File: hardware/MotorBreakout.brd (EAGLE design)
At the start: 160 x 100 mm, 1 part

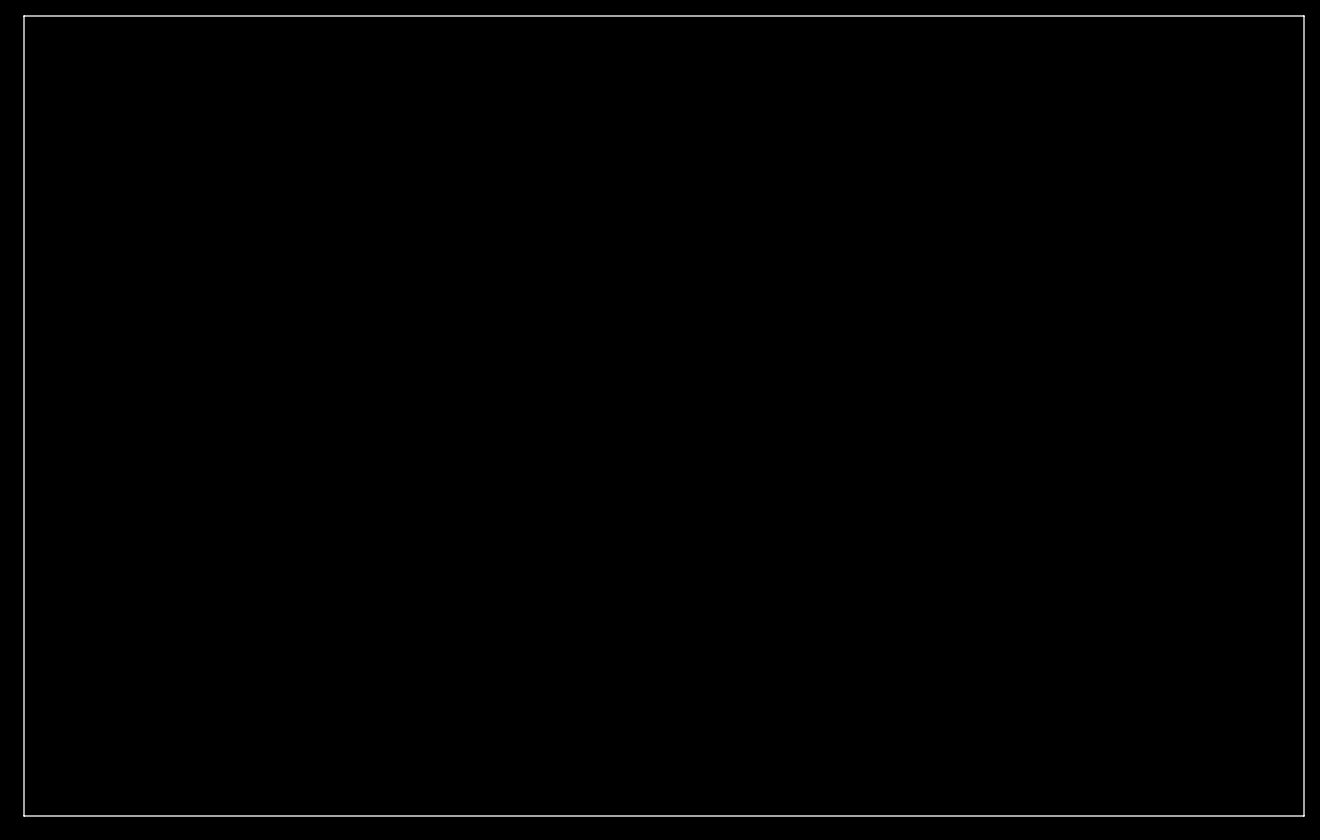
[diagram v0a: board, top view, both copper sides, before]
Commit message: Basic breakout complete.y
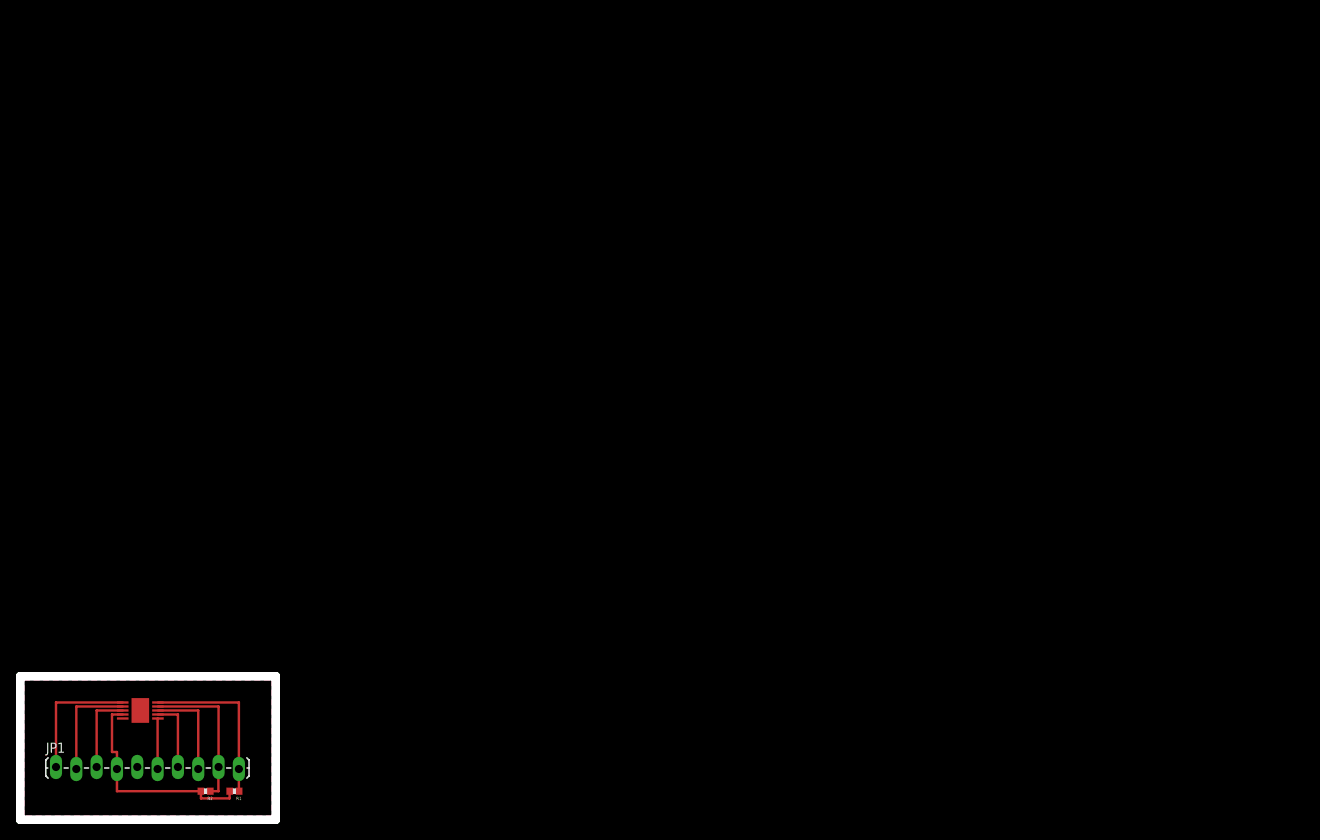
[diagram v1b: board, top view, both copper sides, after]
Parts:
- added JP1: (no value), SparkFun-Connectors:1X10_LOCK_LONGPADS
- added R1, R2: 4.7k, SparkFun-Resistors:0402-RES
- added U$1: DRV8830, DRV8830:DRV8830
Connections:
- new net !FAULT: JP1.6, U$1.P$6
- new net 3.3V: JP1.4, R1.2, R2.2, U$1.P$4
- new net A0: JP1.7, U$1.P$7
- new net A1: JP1.8, U$1.P$8
- new net GND: JP1.5, U$1.P$11, U$1.P$5
- new net ISENSE: JP1.2, U$1.P$2
- new net OUT1: JP1.3, U$1.P$3
- new net OUT2: JP1.1, U$1.P$1
- new net SCL: JP1.10, R1.1, U$1.P$10
- new net SDA: JP1.9, R2.1, U$1.P$9
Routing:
- net 3.3V: track 0.00 -> 27.4 mm
- net SCL: track 0.00 -> 21.2 mm
- net SDA: track 0.00 -> 19.2 mm
- net OUT2: track 0.00 -> 16.4 mm
- net ISENSE: track 0.00 -> 13.6 mm
- net A1: track 0.00 -> 12.4 mm
- net OUT1: track 0.00 -> 10.3 mm
- net A0: track 0.00 -> 9.06 mm
- net !FAULT: track 0.00 -> 6.36 mm
- added copper zone on layer 1, net GND
- added copper zone on layer 16, net GND
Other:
- board size 160 x 100 mm -> 32 x 18 mm
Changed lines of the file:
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@@
 <setting verticaltext="up"/>
 </settings>
-<grid distance="0.05" unitdist="inch" unit="inch" style="lines" multiple="1" display="no" altdistance="0.025" altunitdist="inch" altunit="inch"/>
+<grid distance="0.5" unitdist="mm" unit="mm" style="lines" multiple="1" display="yes" altdistance="0.1" altunitdist="mm" altunit="mm"/>
 <layers>
 <layer number="1" name="Top" color="4" fill="1" visible="yes" active="yes"/>
@@
 <layer number="44" name="Drills" color="7" fill="1" visible="no" active="yes"/>
 <layer number="45" name="Holes" color="7" fill="1" visible="no" active="yes"/>
-<layer number="46" name="Milling" color="3" fill="1" visible="no" active="yes"/>
+<layer number="46" name="Milling" color="3" fill="1" visible="yes" active="yes"/>
 <layer number="47" name="Measures" color="7" fill="1" visible="no" active="yes"/>
 <layer number="48" name="Document" color="7" fill="1" visible="yes" active="yes"/>
@@
 <layer number="113" name="IDFDebug" color="4" fill="1" visible="yes" active="yes"/>
 <layer number="116" name="Patch_BOT" color="9" fill="4" visible="yes" active="yes"/>
+<layer number="118" name="Rect_Pads" color="7" fill="1" visible="yes" active="yes"/>
 <layer number="121" name="_tsilk" color="7" fill="1" visible="yes" active="yes"/>
 <layer number="122" name="_bsilk" color="7" fill="1" visible="yes" active="yes"/>
@@
 <board>
 <plain>
-<wire x1="0" y1="0" x2="160" y2="0" width="0" layer="20"/>
-<wire x1="160" y1="0" x2="160" y2="100" width="0" layer="20"/>
-<wire x1="160" y1="100" x2="0" y2="100" width="0" layer="20"/>
-<wire x1="0" y1="100" x2="0" y2="0" width="0" layer="20"/>
+<wire x1="0" y1="0" x2="31" y2="0" width="0" layer="20"/>
+<wire x1="31" y1="0" x2="31" y2="17" width="0" layer="20"/>
+<wire x1="31" y1="17" x2="0" y2="17" width="0" layer="20"/>
+<wire x1="0" y1="17" x2="0" y2="0" width="0" layer="20"/>
+<wire x1="-0.5" y1="17.5" x2="31.5" y2="17.5" width="1" layer="46"/>
+<wire x1="31.5" y1="17.5" x2="31.5" y2="-0.5" width="1" layer="46"/>
+<wire x1="31.5" y1="-0.5" x2="-0.5" y2="-0.5" width="1" layer="46"/>
+<wire x1="-0.5" y1="-0.5" x2="-0.5" y2="17.5" width="1" layer="46"/>
 </plain>
 <attributes>
@@
 <attribute name="DESIGNER" value="Nobody" x="0" y="0" size="1.778" layer="27" display="off"/>
 </element>
+<element name="U$1" library="DRV8830" package="DRV8830" value="DRV8830" x="14.54" y="13.19"/>
+<element name="JP1" library="SparkFun-Connectors" package="1X10_LOCK_LONGPADS" value="" x="4" y="6"/>
+<element name="R1" library="SparkFun-Resistors" package="0402-RES" value="4.7k" x="26.3" y="3.1" rot="R180"/>
+<element name="R2" library="SparkFun-Resistors" package="0402-RES" value="4.7k" x="22.7" y="3.1" rot="R180"/>
 </elements>
 <signals>
+<signal name="3.3V">
+<contactref element="U$1" pad="P$4"/>
+<contactref element="JP1" pad="4"/>
+<wire x1="12.34" y1="12.69" x2="11" y2="12.69" width="0.3048" layer="1"/>
+<wire x1="11" y1="12.69" x2="11" y2="8" width="0.3048" layer="1"/>
+<wire x1="11" y1="8" x2="11.62" y2="8" width="0.3048" layer="1"/>
+<wire x1="11.62" y1="8" x2="11.62" y2="5.873" width="0.3048" layer="1"/>
+<contactref element="R1" pad="2"/>
+<contactref element="R2" pad="2"/>
+<wire x1="22.12" y1="3.1" x2="11.62" y2="3.1" width="0.3048" layer="1"/>
+<wire x1="11.62" y1="3.1" x2="11.62" y2="5.873" width="0.3048" layer="1"/>
+<wire x1="25.72" y1="3.1" x2="25.7" y2="3.1" width="0.3048" layer="1"/>
+<wire x1="25.7" y1="3.1" x2="25.7" y2="2.2" width="0.3048" layer="1"/>
+<wire x1="25.7" y1="2.2" x2="22.12" y2="2.2" width="0.3048" layer="1"/>
+<wire x1="22.12" y1="2.2" x2="22.12" y2="3.1" width="0.3048" layer="1"/>
+</signal>
+<signal name="GND">
+<contactref element="U$1" pad="P$5"/>
+<polygon width="0.4064" layer="16">
+<vertex x="0" y="17"/>
+<vertex x="31" y="17"/>
+<vertex x="31" y="0"/>
+<vertex x="0" y="0"/>
+</polygon>
+<polygon width="0.4064" layer="1">
+<vertex x="0" y="17"/>
+<vertex x="31" y="17"/>
+<vertex x="31" y="0"/>
+<vertex x="0" y="0"/>
+</polygon>
+<contactref element="U$1" pad="P$11"/>
+<contactref element="JP1" pad="5"/>
+</signal>
+<signal name="OUT1">
+<contactref element="U$1" pad="P$3"/>
+<contactref element="JP1" pad="3"/>
+<wire x1="12.34" y1="13.19" x2="9.08" y2="13.19" width="0.3048" layer="1"/>
+<wire x1="9.08" y1="13.19" x2="9.08" y2="6.127" width="0.3048" layer="1"/>
+</signal>
+<signal name="ISENSE">
+<contactref element="U$1" pad="P$2"/>
+<contactref element="JP1" pad="2"/>
+<wire x1="12.34" y1="13.69" x2="6.54" y2="13.69" width="0.3048" layer="1"/>
+<wire x1="6.54" y1="13.69" x2="6.54" y2="5.873" width="0.3048" layer="1"/>
+</signal>
+<signal name="OUT2">
+<contactref element="U$1" pad="P$1"/>
+<contactref element="JP1" pad="1"/>
+<wire x1="12.34" y1="14.19" x2="4" y2="14.19" width="0.3048" layer="1"/>
+<wire x1="4" y1="14.19" x2="4" y2="6.127" width="0.3048" layer="1"/>
+</signal>
+<signal name="SCL">
+<contactref element="U$1" pad="P$10"/>
+<contactref element="JP1" pad="10"/>
+<wire x1="16.74" y1="14.19" x2="26.86" y2="14.19" width="0.3048" layer="1"/>
+<wire x1="26.86" y1="14.19" x2="26.86" y2="5.873" width="0.3048" layer="1"/>
+<contactref element="R1" pad="1"/>
+<wire x1="26.88" y1="3.1" x2="26.86" y2="3.1" width="0.3048" layer="1"/>
+<wire x1="26.86" y1="3.1" x2="26.86" y2="5.873" width="0.3048" layer="1"/>
+</signal>
+<signal name="SDA">
+<contactref element="U$1" pad="P$9"/>
+<contactref element="JP1" pad="9"/>
+<wire x1="16.74" y1="13.69" x2="24.32" y2="13.69" width="0.3048" layer="1"/>
+<wire x1="24.32" y1="13.69" x2="24.32" y2="6.127" width="0.3048" layer="1"/>
+<contactref element="R2" pad="1"/>
+<wire x1="24.32" y1="6.127" x2="24.3" y2="6.127" width="0.3048" layer="1"/>
+<wire x1="24.3" y1="6.127" x2="24.3" y2="3.1" width="0.3048" layer="1"/>
+<wire x1="24.3" y1="3.1" x2="23.28" y2="3.1" width="0.3048" layer="1"/>
+</signal>
+<signal name="A1">
+<contactref element="U$1" pad="P$8"/>
+<contactref element="JP1" pad="8"/>
+<wire x1="16.74" y1="13.19" x2="21.78" y2="13.19" width="0.3048" layer="1"/>
+<wire x1="21.78" y1="13.19" x2="21.78" y2="5.873" width="0.3048" layer="1"/>
+</signal>
+<signal name="A0">
+<contactref element="U$1" pad="P$7"/>
+<contactref element="JP1" pad="7"/>
+<wire x1="16.74" y1="12.69" x2="19.24" y2="12.69" width="0.3048" layer="1"/>
+<wire x1="19.24" y1="12.69" x2="19.24" y2="6.127" width="0.3048" layer="1"/>
+</signal>
+<signal name="!FAULT">
+<contactref element="U$1" pad="P$6"/>
+<contactref element="JP1" pad="6"/>
+<wire x1="16.74" y1="12.19" x2="16.7" y2="12.19" width="0.3048" layer="1"/>
+<wire x1="16.7" y1="12.19" x2="16.7" y2="5.873" width="0.3048" layer="1"/>
+</signal>
 </signals>
 </board>
